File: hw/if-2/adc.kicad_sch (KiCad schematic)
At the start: 20 parts, among them J4 Conn_01x02, U3 PCM1804DBR

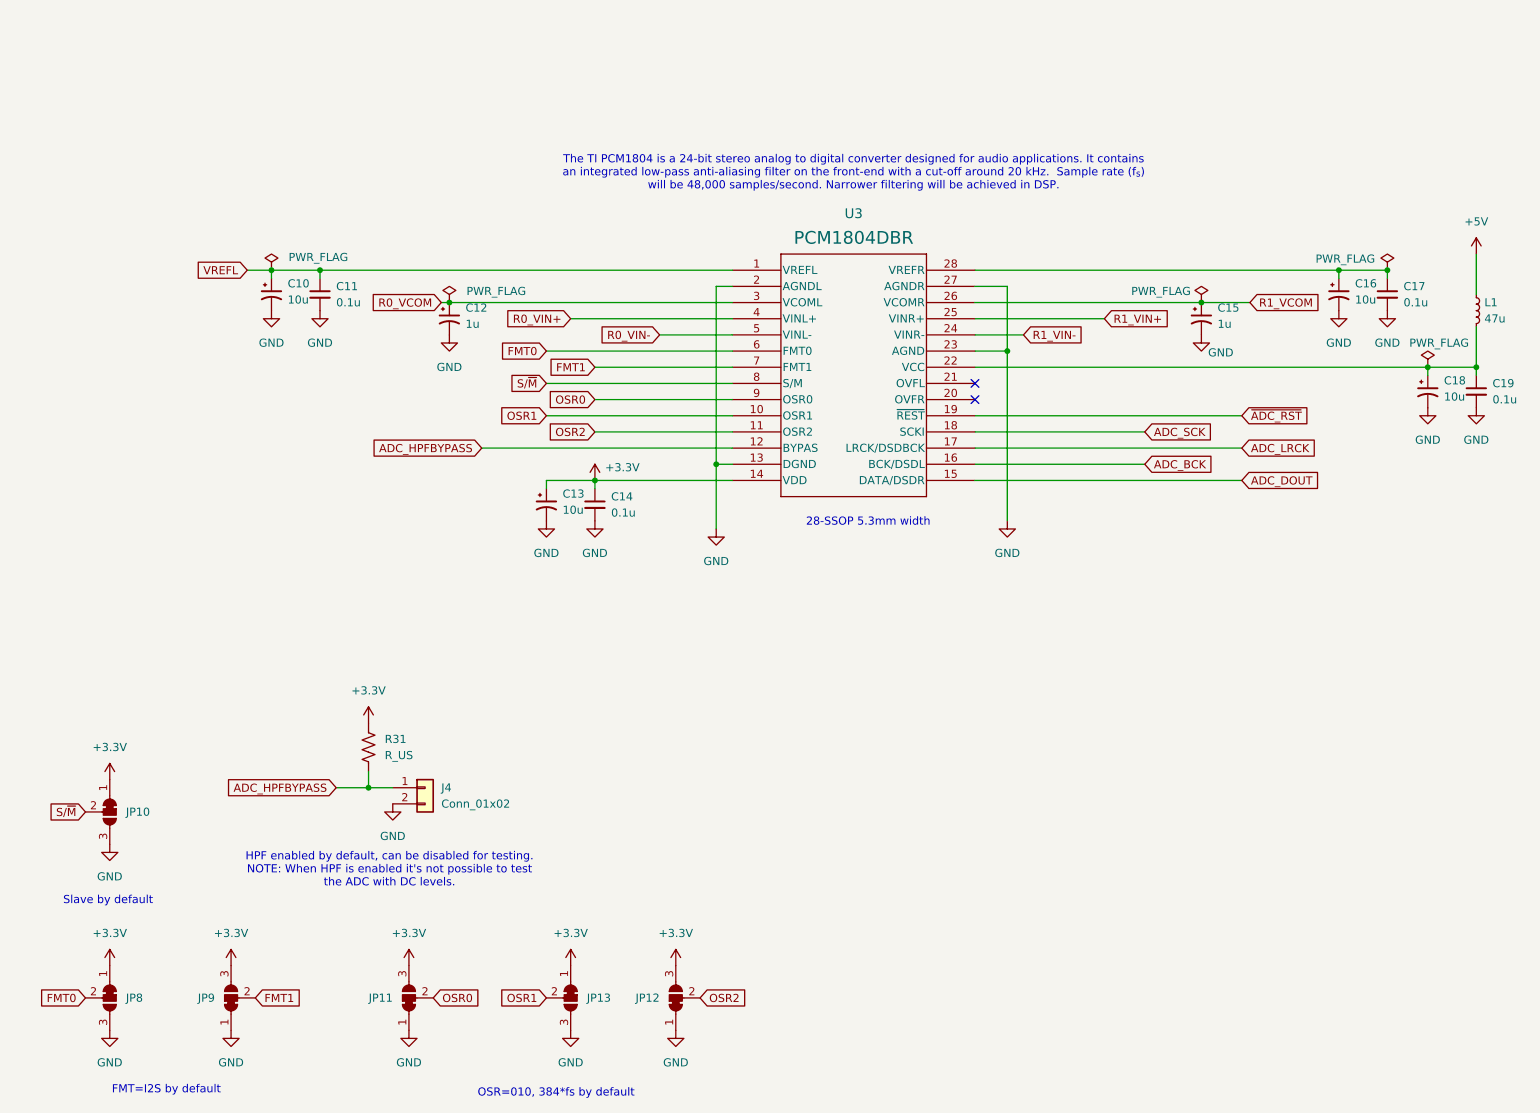
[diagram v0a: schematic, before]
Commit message: First draft of schematic
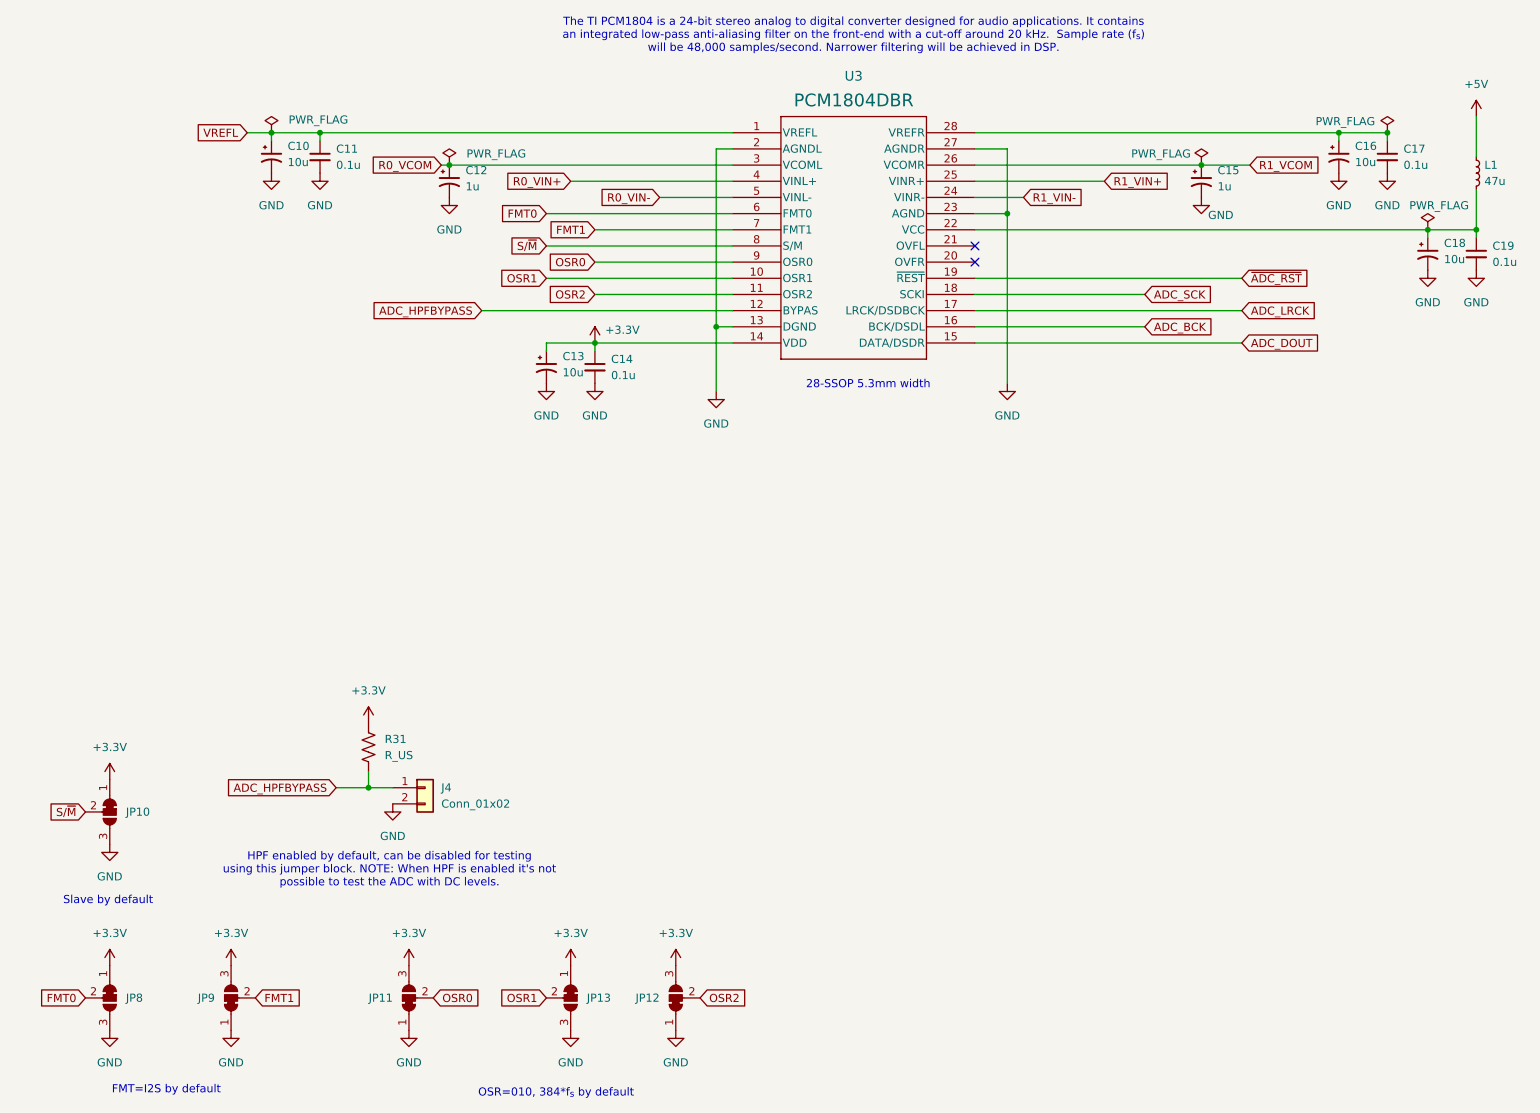
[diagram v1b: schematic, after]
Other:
- note added: "HPF enabled by default, can be disabled for testing using this jumper block. NOTE: When HPF is enabled it's not possible to test the ADC with DC levels."
- note added: "OSR=010, 384*f_{s} by default"
- note removed: "HPF enabled by default, can be disabled for testing. NOTE: When HPF is enabled it's not possible to test the ADC with DC levels."
- note removed: "OSR=010, 384*fs by default"
- moved on the sheet: C10, C11, C12, C13, C14, C15, C16, C17, C18, C19, L1, U3
